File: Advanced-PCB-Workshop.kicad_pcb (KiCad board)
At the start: 2 copper layers, 39.9 x 39.5 mm, 36 parts, among them J1 USB_C_Receptacle_USB2.0_14P, J2 Conn_01x03_Pin, J3 Conn_01x14_Socket, J4 Conn_01x14_Socket, SW1 SW_Nidec_CAS-120A1, SW2 SW_Push, U1 RP2040, U2 W25Q128JVS, U3 AMS1117-3.3, Y1 ABM8-272-T3

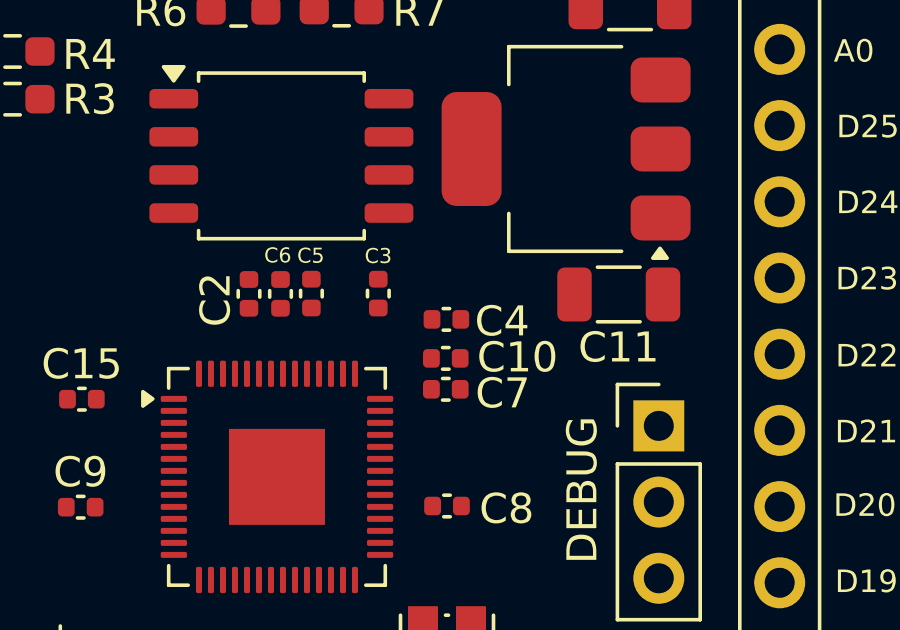
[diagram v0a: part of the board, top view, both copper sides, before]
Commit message: Final Template v1.3.0
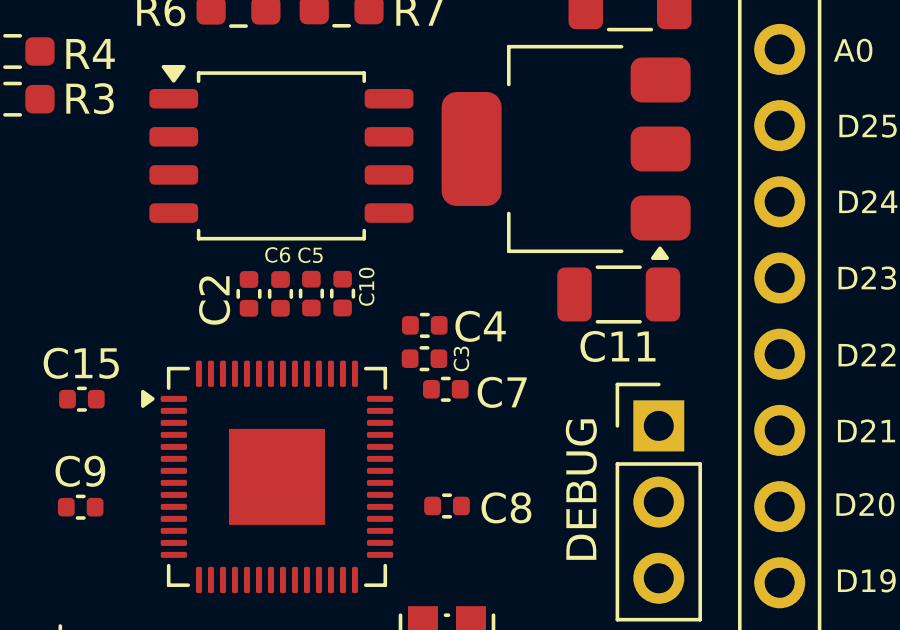
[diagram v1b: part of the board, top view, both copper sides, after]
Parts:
- moved C10 4.06 mm to (134.2, 105.2), turned to -90 degrees
- moved C3 2.66 mm to (136.9, 107.3), turned to 180 degrees
- moved C4 0.75 mm to (136.9, 106.2)
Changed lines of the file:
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@@
 	(footprint "Capacitor_SMD:C_0402_1005Metric"
 		(layer "F.Cu")
-		(at 135.35 105.18 -90)
+		(at 136.89 107.35 180)
 		(descr "Capacitor SMD 0402 (1005 Metric), square (rectangular) end terminal, IPC-7351 nominal, (Body size source: IPC-SM-782 page 76, https://www.pcb-3d.com/wordpress/wp-content/uploads/ipc-sm-782a_amendment_1_and_2.pdf), generated with kicad-footprint-generator")
 		(tags "capacitor")
 		(property "Reference" "C3"
-			(at -1.25 0 0)
+			(at -1.25 0 90)
 			(layer "F.SilkS")
 			(effects
@@
 		)
 		(property "Value" "1uF"
-			(at 0 1.16 90)
+			(at 0 1.16 0)
 			(layer "F.Fab")
 			(effects
@@
 		)
 		(property "Datasheet" "https://www.mouser.com/datasheet/2/396/mlcc02_e-1307760.pdf"
-			(at 0 0 90)
+			(at 0 0 0)
 			(layer "F.Fab")
 			(hide yes)
@@
 		)
 		(property "Description" "Unpolarized capacitor"
-			(at 0 0 90)
+			(at 0 0 0)
 			(layer "F.Fab")
 			(hide yes)
@@
 		)
 		(fp_line
-			(start -0.91 0.46)
-			(end -0.91 -0.46)
+			(start 0.91 0.46)
+			(end -0.91 0.46)
 			(stroke
 				(width 0.05)
@@
 		)
 		(fp_line
-			(start 0.91 0.46)
-			(end -0.91 0.46)
+			(start 0.91 -0.46)
+			(end 0.91 0.46)
 			(stroke
 				(width 0.05)
@@
 		)
 		(fp_line
-			(start -0.91 -0.46)
-			(end 0.91 -0.46)
+			(start -0.91 0.46)
+			(end -0.91 -0.46)
 			(stroke
 				(width 0.05)
@@
 		)
 		(fp_line
-			(start 0.91 -0.46)
-			(end 0.91 0.46)
+			(start -0.91 -0.46)
+			(end 0.91 -0.46)
 			(stroke
 				(width 0.05)
@@
 		)
 		(fp_line
-			(start -0.5 0.25)
-			(end -0.5 -0.25)
+			(start 0.5 0.25)
+			(end -0.5 0.25)
 			(stroke
 				(width 0.1)
@@
 		)
 		(fp_line
-			(start 0.5 0.25)
-			(end -0.5 0.25)
+			(start 0.5 -0.25)
+			(end 0.5 0.25)
 			(stroke
 				(width 0.1)
@@
 		)
 		(fp_line
-			(start -0.5 -0.25)
-			(end 0.5 -0.25)
+			(start -0.5 0.25)
+			(end -0.5 -0.25)
 			(stroke
 				(width 0.1)
@@
 		)
 		(fp_line
-			(start 0.5 -0.25)
-			(end 0.5 0.25)
+			(start -0.5 -0.25)
+			(end 0.5 -0.25)
 			(stroke
 				(width 0.1)
@@
 		)
 		(fp_text user "${REFERENCE}"
-			(at 0 0 90)
+			(at 0 0 0)
 			(layer "F.Fab")
 			(effects
@@
 		)
 		(pad "1" smd roundrect
-			(at -0.48 0 270)
+			(at -0.48 0 180)
 			(size 0.56 0.62)
 			(layers "F.Cu" "F.Mask" "F.Paste")
@@
 		)
 		(pad "2" smd roundrect
-			(at 0.48 0 270)
+			(at 0.48 0 180)
 			(size 0.56 0.62)
 			(layers "F.Cu" "F.Mask" "F.Paste")
@@
 	(footprint "Capacitor_SMD:C_0402_1005Metric"
 		(layer "F.Cu")
-		(at 137.62 106.04 180)
+		(at 136.9 106.24 180)
 		(descr "Capacitor SMD 0402 (1005 Metric), square (rectangular) end terminal, IPC-7351 nominal, (Body size source: IPC-SM-782 page 76, https://www.pcb-3d.com/wordpress/wp-content/uploads/ipc-sm-782a_amendment_1_and_2.pdf), generated with kicad-footprint-generator")
 		(tags "capacitor")
@@
 	(footprint "Capacitor_SMD:C_0402_1005Metric"
 		(layer "F.Cu")
-		(at 137.6 107.34 180)
+		(at 134.16 105.18 -90)
 		(descr "Capacitor SMD 0402 (1005 Metric), square (rectangular) end terminal, IPC-7351 nominal, (Body size source: IPC-SM-782 page 76, https://www.pcb-3d.com/wordpress/wp-content/uploads/ipc-sm-782a_amendment_1_and_2.pdf), generated with kicad-footprint-generator")
 		(tags "capacitor")
 		(property "Reference" "C10"
-			(at -2.39 0.03 180)
+			(at -0.23 -0.82 90)
 			(layer "F.SilkS")
 			(effects
 				(font
-					(size 1 1)
-					(thickness 0.15)
+					(size 0.5 0.5)
+					(thickness 0.125)
 				)
 			)
 		)
 		(property "Value" "100nF"
-			(at 0 1.16 180)
+			(at 0 1.16 90)
 			(layer "F.Fab")
 			(effects
@@
 		)
 		(property "Datasheet" "https://www.mouser.com/ProductDetail/KYOCERA-AVX/KGM02AR51A104MH?qs=9vOqFld9vZUKqUoT7PZO0Q%3D%3D"
-			(at 0 0 180)
+			(at 0 0 90)
 			(layer "F.Fab")
 			(hide yes)
@@
 		)
 		(property "Description" "Unpolarized capacitor"
-			(at 0 0 180)
+			(at 0 0 90)
 			(layer "F.Fab")
 			(hide yes)
@@
 		)
 		(fp_line
-			(start 0.91 0.46)
-			(end -0.91 0.46)
+			(start -0.91 0.46)
+			(end -0.91 -0.46)
 			(stroke
 				(width 0.05)
@@
 		)
 		(fp_line
-			(start 0.91 -0.46)
-			(end 0.91 0.46)
+			(start 0.91 0.46)
+			(end -0.91 0.46)
 			(stroke
 				(width 0.05)
@@
 		)
 		(fp_line
-			(start -0.91 0.46)
-			(end -0.91 -0.46)
+			(start -0.91 -0.46)
+			(end 0.91 -0.46)
 			(stroke
 				(width 0.05)
@@
 		)
 		(fp_line
-			(start -0.91 -0.46)
-			(end 0.91 -0.46)
+			(start 0.91 -0.46)
+			(end 0.91 0.46)
 			(stroke
 				(width 0.05)
@@
 		)
 		(fp_line
-			(start 0.5 0.25)
-			(end -0.5 0.25)
+			(start -0.5 0.25)
+			(end -0.5 -0.25)
 			(stroke
 				(width 0.1)
@@
 		)
 		(fp_line
-			(start 0.5 -0.25)
-			(end 0.5 0.25)
+			(start 0.5 0.25)
+			(end -0.5 0.25)
 			(stroke
 				(width 0.1)
@@
 		)
 		(fp_line
-			(start -0.5 0.25)
-			(end -0.5 -0.25)
+			(start -0.5 -0.25)
+			(end 0.5 -0.25)
 			(stroke
 				(width 0.1)
@@
 		)
 		(fp_line
-			(start -0.5 -0.25)
-			(end 0.5 -0.25)
+			(start 0.5 -0.25)
+			(end 0.5 0.25)
 			(stroke
 				(width 0.1)
@@
 		)
 		(fp_text user "${REFERENCE}"
-			(at 0 0 180)
+			(at 0 0 90)
 			(layer "F.Fab")
 			(effects
@@
 		)
 		(pad "1" smd roundrect
-			(at -0.48 0 180)
+			(at -0.48 0 270)
 			(size 0.56 0.62)
 			(layers "F.Cu" "F.Mask" "F.Paste")
@@
 		)
 		(pad "2" smd roundrect
-			(at 0.48 0 180)
+			(at 0.48 0 270)
 			(size 0.56 0.62)
 			(layers "F.Cu" "F.Mask" "F.Paste")
